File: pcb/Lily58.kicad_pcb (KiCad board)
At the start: 2 copper layers, 142.5 x 106.3 mm, 88 parts, among them J1 LED, J2 4PIN, P1 i2c_pin, P2 i2c_pin, P3 ICSP, SW1 SW_PUSH, SW10 SW_PUSH, SW11 SW_PUSH, SW12 SW_PUSH, SW13 SW_PUSH, SW14 SW_PUSH, SW15 SW_PUSH, SW16 SW_PUSH, SW17 SW_PUSH, SW18 SW_PUSH, SW19 SW_PUSH, SW2 SW_PUSH, SW20 SW_PUSH, SW21 SW_PUSH, SW22 SW_PUSH, SW23 SW_PUSH, SW24 SW_PUSH, SW25 SW_PUSH, SW26 SW_PUSH, SW27 SW_PUSH, SW28 SW_PUSH, SW29 SW_PUSH, SW3 SW_PUSH, SW4 SW_PUSH, SW5 SW_PUSH, SW6 SW_PUSH, SW7 SW_PUSH, SW8 SW_PUSH, SW9 SW_PUSH, U1 ProMicro

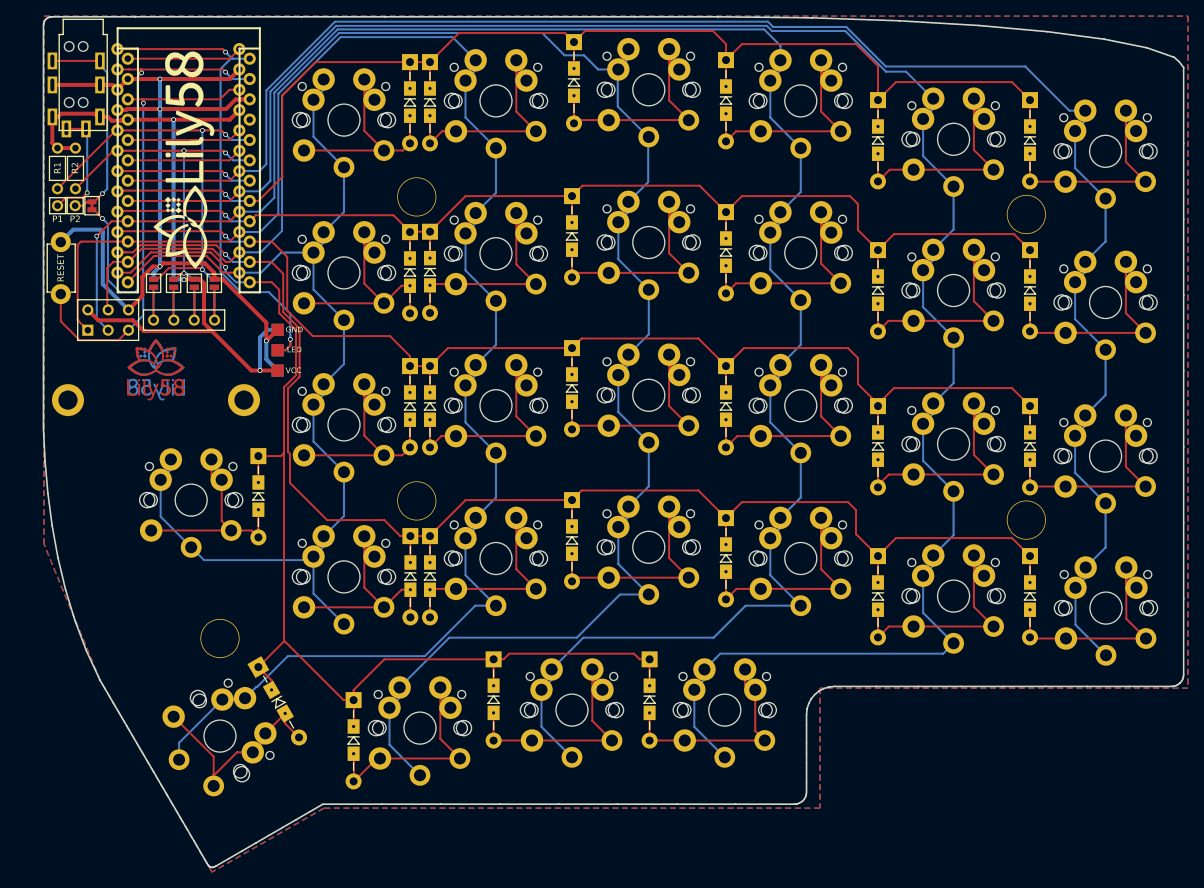
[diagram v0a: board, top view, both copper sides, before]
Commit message: First version for prototyping
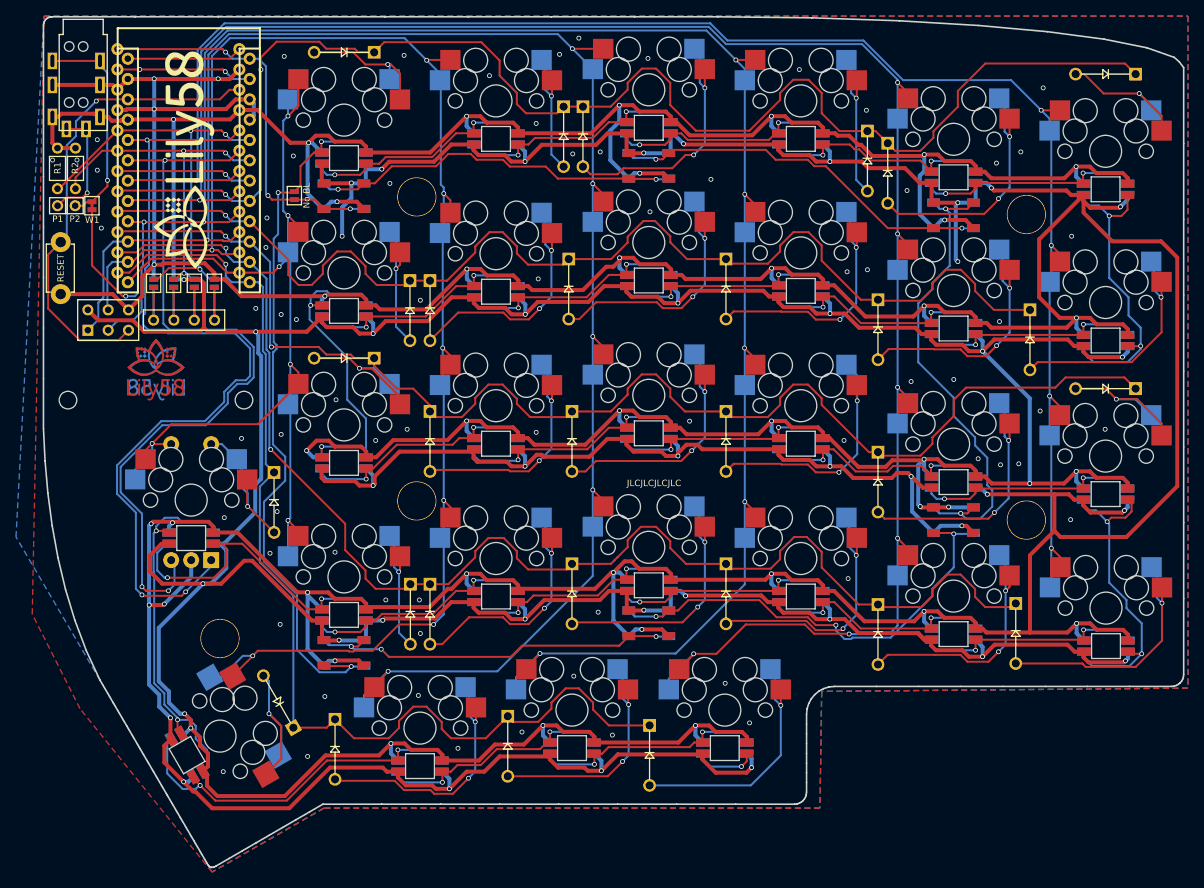
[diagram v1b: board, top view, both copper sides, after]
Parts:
- removed the J1 at (112.2, 81.3)
- added D30: WS2812B, Lily58-footprint:WS2812B-double sided, F.Cu at (120.5, 59.5)
- added D31: WS2812B, Lily58-footprint:WS2812B-double sided, F.Cu at (158.6, 55.7)
- added D32: WS2812B, Lily58-footprint:WS2812B-double sided, F.Cu at (196.7, 61.9)
- added D33: WS2812B, Lily58-footprint:WS2812B-double sided, F.Cu at (120.5, 116.6)
- added D34: WS2812B, Lily58-footprint:WS2812B-double sided, F.Cu at (158.6, 112.9)
- added D35: WS2812B, Lily58-footprint:WS2812B-double sided, F.Cu at (196.7, 100.0)
- added JP1: Jumper_NO_Small, Lily58-footprint:Jumper, F.Cu at (114.3, 59.4)
- added LED1: YS-SK6812MINI-E, Lily58-footprint:SK6812MINI-E, F.Cu at (120.5, 54.8)
- added LED10: YS-SK6812MINI-E, Lily58-footprint:SK6812MINI-E, F.Cu at (177.6, 71.3)
- added LED11: YS-SK6812MINI-E, Lily58-footprint:SK6812MINI-E, F.Cu at (196.7, 76.0)
- added LED12: YS-SK6812MINI-E, Lily58-footprint:SK6812MINI-E, F.Cu at (215.7, 77.5)
- added LED13: YS-SK6812MINI-E, Lily58-footprint:SK6812MINI-E, F.Cu at (120.5, 92.8)
- added LED14: YS-SK6812MINI-E, Lily58-footprint:SK6812MINI-E, F.Cu at (139.5, 90.5)
- added LED15: YS-SK6812MINI-E, Lily58-footprint:SK6812MINI-E, F.Cu at (158.6, 89.2)
- added LED16: YS-SK6812MINI-E, Lily58-footprint:SK6812MINI-E, F.Cu at (177.6, 90.5)
- added LED17: YS-SK6812MINI-E, Lily58-footprint:SK6812MINI-E, F.Cu at (196.7, 95.2)
- added LED18: YS-SK6812MINI-E, Lily58-footprint:SK6812MINI-E, F.Cu at (215.7, 96.8)
- added LED19: YS-SK6812MINI-E, Lily58-footprint:SK6812MINI-E, F.Cu at (120.5, 111.8)
- added LED2: YS-SK6812MINI-E, Lily58-footprint:SK6812MINI-E, F.Cu at (139.5, 52.4)
- added LED20: YS-SK6812MINI-E, Lily58-footprint:SK6812MINI-E, F.Cu at (139.5, 109.5)
- added LED21: YS-SK6812MINI-E, Lily58-footprint:SK6812MINI-E, F.Cu at (158.6, 108.2)
- added LED22: YS-SK6812MINI-E, Lily58-footprint:SK6812MINI-E, F.Cu at (177.6, 109.5)
- added LED23: YS-SK6812MINI-E, Lily58-footprint:SK6812MINI-E, F.Cu at (196.7, 114.2)
- added LED24: YS-SK6812MINI-E, Lily58-footprint:SK6812MINI-E, F.Cu at (215.8, 115.8)
- added LED25: YS-SK6812MINI-E, Lily58-footprint:SK6812MINI-E, F.Cu at (101.4, 102.2)
- added LED26: YS-SK6812MINI-E, Lily58-footprint:SK6812MINI-E, F.Cu at (100.9, 129.4)
- added LED27: YS-SK6812MINI-E, Lily58-footprint:SK6812MINI-E, F.Cu at (130.0, 130.8)
- added LED28: YS-SK6812MINI-E, Lily58-footprint:SK6812MINI-E, F.Cu at (149.0, 128.5)
- added LED29: YS-SK6812MINI-E, Lily58-footprint:SK6812MINI-E, F.Cu at (168.1, 128.5)
- added LED3: YS-SK6812MINI-E, Lily58-footprint:SK6812MINI-E, F.Cu at (158.6, 51.0)
- added LED4: YS-SK6812MINI-E, Lily58-footprint:SK6812MINI-E, F.Cu at (177.6, 52.4)
- added LED5: YS-SK6812MINI-E, Lily58-footprint:SK6812MINI-E, F.Cu at (196.7, 57.1)
- added LED6: YS-SK6812MINI-E, Lily58-footprint:SK6812MINI-E, F.Cu at (215.7, 58.6)
- added LED7: YS-SK6812MINI-E, Lily58-footprint:SK6812MINI-E, F.Cu at (120.5, 73.8)
- added LED8: YS-SK6812MINI-E, Lily58-footprint:SK6812MINI-E, F.Cu at (139.5, 71.5)
- added LED9: YS-SK6812MINI-E, Lily58-footprint:SK6812MINI-E, F.Cu at (158.6, 70.0)
- added SW30: RotaryEncoder_Switch, Lily58-footprint:RotaryEncoder_EC11-no-legs_noSS, B.Cu at (101.4, 97.5)
- D1, D10, D11, D12, D13, D14, D15, D16, D17, D18, D19, D2, D20, D21, D22, D23, D24, D25, D26, D27, D28, D29, D3, D4, D5, D6, D7, D8, D9: footprint Lily58-footprint:Diode_TH_SOD123 -> Lily58-footprint:Diode-Doublesided-TH-7.5mm
- JP2: renamed from JP1; value (none) -> Jumper_NO_Small
- JP3: renamed from JP2; value (none) -> Jumper_NO_Small
- JP4: renamed from JP3; value (none) -> Jumper_NO_Small
- JP5: renamed from JP4; value (none) -> Jumper_NO_Small
- JP6: renamed from JP5; value (none) -> Jumper_NO_Small
- JP7: renamed from JP6; value (none) -> Jumper_NO_Small
- JP8: renamed from JP7; value (none) -> Jumper_NO_Small
- JP9: renamed from JP8; value (none) -> Jumper_NO_Small
- SW1, SW10, SW11, SW12, SW13, SW14, SW15, SW16, SW17, SW18, SW19, SW2, SW20, SW21, SW22, SW23, SW24, SW25, SW27, SW28, SW29, SW3, SW4, SW5, SW6, SW7, SW8, SW9: footprint Lily58-footprint:MX_PG1350-Under_FLIP_HOLES_18mm -> Lily58-footprint:MX_Socket_18mm
- SW26: footprint Lily58-footprint:MX_PG1350-Under_FLIP_HOLES_27mm -> Lily58-footprint:MX_Socket_18mm
- TH1, TH2: footprint Lily58-footprint:M2_HOLE_PCB -> Lily58-footprint:HOLE_M2
- moved D4 19.2 mm to (185.9, 55.1), turned to 90 degrees
- moved D2 17.3 mm to (148.0, 52.1), turned to 90 degrees
- moved D6 12.5 mm to (215.7, 44.2), turned to 0 degrees
- moved D18 11.9 mm to (215.7, 83.6), turned to 0 degrees
- moved D1 10.3 mm to (120.5, 41.5), turned to 0 degrees
- moved D13 10.2 mm to (120.5, 79.8), turned to 0 degrees
- moved D29 7.01 mm to (158.7, 129.4), turned to 90 degrees
- moved D3 6.91 mm to (150.4, 52.1), turned to 90 degrees
- moved D21 6.72 mm to (149.0, 109.2), turned to 90 degrees
- moved D15 6.67 mm to (149.0, 90.2), turned to 90 degrees
- moved D9 6.63 mm to (148.6, 71.1), turned to 90 degrees
- moved D12 6.22 mm to (206.2, 77.5), turned to 90 degrees
- moved D28 6.13 mm to (141.0, 128.3), turned to 90 degrees
- moved D24 5.00 mm to (204.5, 114.2), turned to 90 degrees
- moved D11 4.95 mm to (187.2, 76.2), turned to 90 degrees
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- renumbered J2 to J1, OLED to P4
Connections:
- U1 pad 19: Net-(U1-Pad19) -> ENCB
- U1 pad 20: Net-(U1-Pad20) -> ENCA
- U1 pad 24: Net-(U1-Pad24) -> unconnected-(U1-Pad24)
- U1 pad 7: Net-(U1-Pad7) -> unconnected-(U1-Pad7)
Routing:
- net GND: track 117.4 -> 940.5 mm, vias 4 -> 117
- net VCC: track 94.8 -> 890.0 mm, vias 3 -> 41
- net ENCA: track 0.00 -> 106.5 mm, vias 0 -> 3
- net ENCB: track 0.00 -> 97.2 mm, vias 0 -> 3
- net Underglow_out: track 0.00 -> 91.3 mm, vias 0 -> 3
- net Net-(D32-Pad2): track 0.00 -> 59.0 mm, vias 0 -> 2
- net Net-(D34-Pad4): track 0.00 -> 57.7 mm, vias 0 -> 3
- net Net-(D31-Pad2): track 0.00 -> 48.0 mm, vias 0 -> 2
- net Net-(D33-Pad4): track 0.00 -> 47.0 mm, vias 0 -> 3
- net Net-(LED25-Pad2): track 0.00 -> 46.9 mm, vias 0 -> 2
- net Net-(D30-Pad2): track 0.00 -> 46.6 mm, vias 0 -> 2
- net Net-(LED26-Pad2): track 0.00 -> 46.5 mm, vias 0 -> 2
- net Net-(LED19-Pad2): track 0.00 -> 42.7 mm, vias 0 -> 2
- net Net-(LED13-Pad4): track 0.00 -> 40.6 mm, vias 0 -> 2
- net Net-(LED18-Pad2): track 0.00 -> 39.0 mm, vias 0 -> 2
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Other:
- net class Default removed
- net class GND removed
- net class VCC removed
- rule pad_to_mask_clearance: 0.2 -> 0
- board text added: "JLCJLCJLCJLC"
- board text added: "No BL"
- board text added: "PCB Design by F_YUUCHI, modified by JeJeff"
- board text removed: "GND"
- board text removed: "LED"
- board text removed: "PCB Design by F_YUUCHI"
- board text removed: "VCC"

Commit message: Revert non-ultra changes from "First version for prototyping"
This partially reverts commit a3e54aa417d9b9a440498bf4f6e0d923b4cb8ab2.
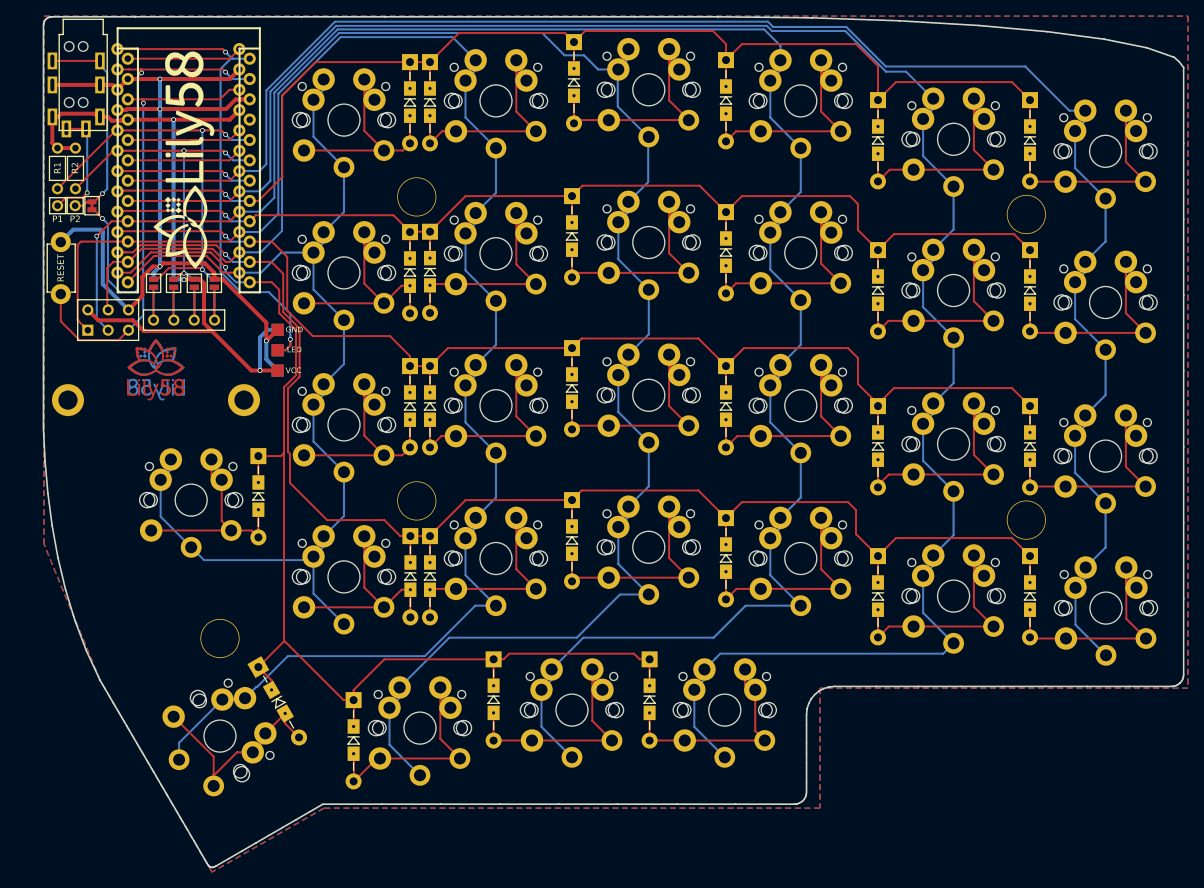
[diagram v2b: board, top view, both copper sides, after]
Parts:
- removed D30, D31, D32, D33, D34, D35: WS2812B, Lily58-footprint:WS2812B-double sided
- removed the JP1 at (114.3, 59.4)
- removed LED1, LED10, LED11, LED12, LED13, LED14, LED15, LED16, LED17, LED18, LED19, LED2, LED20, LED21, LED22, LED23, LED24, LED25, LED26, LED27, LED28, LED29, LED3, LED4, LED5, LED6, LED7, LED8, LED9: YS-SK6812MINI-E, Lily58-footprint:SK6812MINI-E
- removed SW30: RotaryEncoder_Switch, Lily58-footprint:RotaryEncoder_EC11-no-legs_noSS
- added J1: LED, Lily58-footprint:StripLED, F.Cu at (112.2, 81.3)
- D1, D10, D11, D12, D13, D14, D15, D16, D17, D18, D19, D2, D20, D21, D22, D23, D24, D25, D26, D27, D28, D29, D3, D4, D5, D6, D7, D8, D9: footprint Lily58-footprint:Diode-Doublesided-TH-7.5mm -> Lily58-footprint:Diode_TH_SOD123
- JP1: renamed from JP2; value Jumper_NO_Small -> (none)
- JP2: renamed from JP3; value Jumper_NO_Small -> (none)
- JP3: renamed from JP4; value Jumper_NO_Small -> (none)
- JP4: renamed from JP5; value Jumper_NO_Small -> (none)
- JP5: renamed from JP6; value Jumper_NO_Small -> (none)
- JP6: renamed from JP7; value Jumper_NO_Small -> (none)
- JP7: renamed from JP8; value Jumper_NO_Small -> (none)
- JP8: renamed from JP9; value Jumper_NO_Small -> (none)
- SW1, SW10, SW11, SW12, SW13, SW14, SW15, SW16, SW17, SW18, SW19, SW2, SW20, SW21, SW22, SW23, SW24, SW25, SW27, SW28, SW29, SW3, SW4, SW5, SW6, SW7, SW8, SW9: footprint Lily58-footprint:MX_Socket_18mm -> Lily58-footprint:MX_PG1350-Under_FLIP_HOLES_18mm
- SW26: footprint Lily58-footprint:MX_Socket_18mm -> Lily58-footprint:MX_PG1350-Under_FLIP_HOLES_27mm
- TH1, TH2: footprint Lily58-footprint:HOLE_M2 -> Lily58-footprint:M2_HOLE_PCB
- moved D4 19.2 mm to (168.2, 47.5), turned to 270 degrees
- moved D2 17.3 mm to (131.2, 47.8), turned to 270 degrees
- moved D6 12.5 mm to (206.2, 52.5), turned to 270 degrees
- moved D18 11.9 mm to (206.2, 90.8), turned to 270 degrees
- moved D1 10.3 mm to (128.8, 47.8), turned to 270 degrees
- moved D13 10.2 mm to (128.8, 85.8), turned to 270 degrees
- moved D29 7.01 mm to (158.7, 122.4), turned to 270 degrees
- moved D3 6.91 mm to (149.2, 45.2), turned to 270 degrees
- moved D21 6.72 mm to (149.0, 102.5), turned to 270 degrees
- moved D15 6.67 mm to (149.0, 83.5), turned to 270 degrees
- moved D9 6.63 mm to (149.0, 64.5), turned to 270 degrees
- moved D12 6.22 mm to (206.2, 71.2), turned to 270 degrees
- moved D28 6.13 mm to (139.2, 122.4), turned to 270 degrees
- moved D24 5.00 mm to (206.2, 109.5), turned to 270 degrees
- moved D11 4.95 mm to (187.2, 71.2), turned to 270 degrees
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- renumbered J1 to J2, P4 to OLED
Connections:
- U1 pad 19: ENCB -> Net-(U1-Pad19)
- U1 pad 20: ENCA -> Net-(U1-Pad20)
- U1 pad 24: unconnected-(U1-Pad24) -> Net-(U1-Pad24)
- U1 pad 7: unconnected-(U1-Pad7) -> Net-(U1-Pad7)
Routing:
- net GND: track 940.5 -> 117.4 mm, vias 117 -> 4
- net VCC: track 890.0 -> 94.8 mm, vias 41 -> 3
- net ENCA: track 106.5 -> 0.00 mm, vias 3 -> 0
- net ENCB: track 97.2 -> 0.00 mm, vias 3 -> 0
- net Underglow_out: track 91.3 -> 0.00 mm, vias 3 -> 0
- net Net-(D32-Pad2): track 59.0 -> 0.00 mm, vias 2 -> 0
- net Net-(D34-Pad4): track 57.7 -> 0.00 mm, vias 3 -> 0
- net Net-(D31-Pad2): track 48.0 -> 0.00 mm, vias 2 -> 0
- net Net-(D33-Pad4): track 47.0 -> 0.00 mm, vias 3 -> 0
- net Net-(LED25-Pad2): track 46.9 -> 0.00 mm, vias 2 -> 0
- net Net-(D30-Pad2): track 46.6 -> 0.00 mm, vias 2 -> 0
- net Net-(LED26-Pad2): track 46.5 -> 0.00 mm, vias 2 -> 0
- net Net-(LED19-Pad2): track 42.7 -> 0.00 mm, vias 2 -> 0
- net Net-(LED13-Pad4): track 40.6 -> 0.00 mm, vias 2 -> 0
- net Net-(LED18-Pad2): track 39.0 -> 0.00 mm, vias 2 -> 0
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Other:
- net class Default added: clearance 0.2, trace_width 0.25, via_dia 0.6, via_drill 0.4
- net class GND added: clearance 0.2, trace_width 0.5, via_dia 0.6, via_drill 0.4
- net class VCC added: clearance 0.2, trace_width 0.5, via_dia 0.6, via_drill 0.4
- rule pad_to_mask_clearance: 0 -> 0.2
- board text added: "GND"
- board text added: "LED"
- board text added: "PCB Design by F_YUUCHI"
- board text added: "VCC"
- board text removed: "JLCJLCJLCJLC"
- board text removed: "No BL"
- board text removed: "PCB Design by F_YUUCHI, modified by JeJeff"
